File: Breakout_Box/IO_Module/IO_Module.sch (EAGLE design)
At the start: 5 parts, among them U1 AGND, U2 AGND, U3 AGND

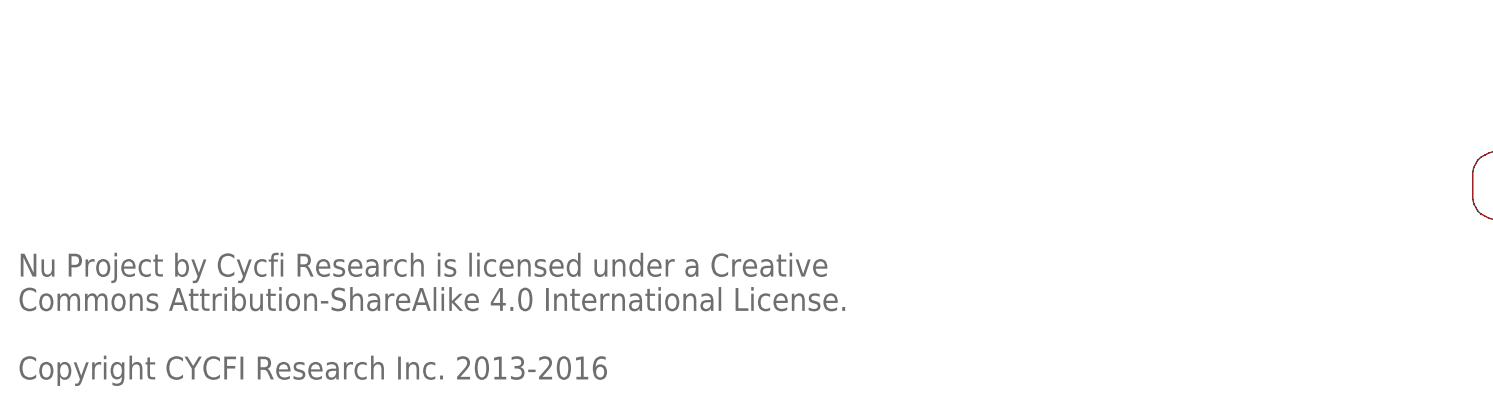
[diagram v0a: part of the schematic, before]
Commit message: Licenses
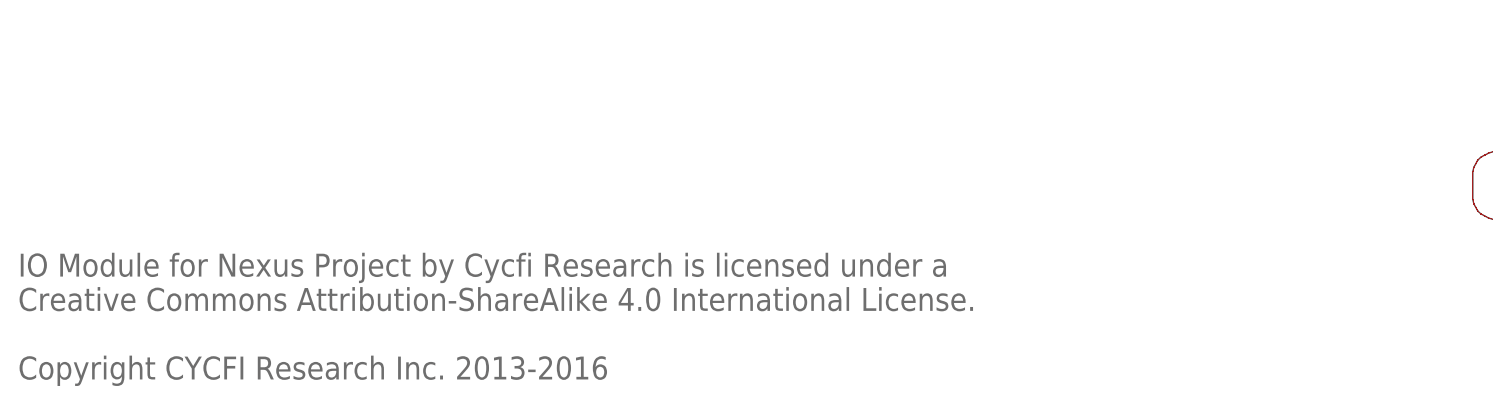
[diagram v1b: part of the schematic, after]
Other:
- note added: "IO Module for Nexus Project by Cycfi Research is licensed under a Creative Commons Attribution-ShareAlike 4.0 International License. Copyright CYCFI Research Inc. 2013-2016"
- note removed: "Nu Project by Cycfi Research is licensed under a Creative Commons Attribution-ShareAlike 4.0 International License. Copyright CYCFI Research Inc. 2013-2016"
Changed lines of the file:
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@@
 <wire x1="233.45903125" y1="25.186403125" x2="233.45903125" y2="33.142509375" width="0" layer="94"/>
 <text x="252.73" y="6.985" size="2.54" layer="95">v0.9</text>
-<text x="12.7" y="7.62" size="2.54" layer="95">Nu Project by Cycfi Research is licensed under a Creative
-Commons Attribution-ShareAlike 4.0 International License.
+<text x="12.7" y="7.62" size="2.54" layer="95">IO Module for Nexus Project by Cycfi Research is licensed under a
+Creative Commons Attribution-ShareAlike 4.0 International License.
 Copyright CYCFI Research Inc. 2013-2016</text>
 <text x="200.025" y="11.43" size="2.54" layer="95">2016050</text>

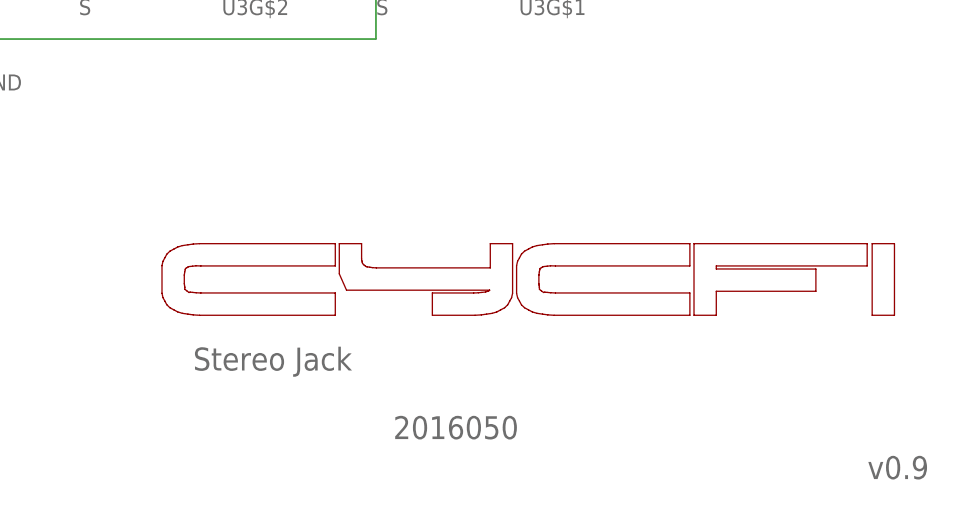
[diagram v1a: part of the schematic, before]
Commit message: *Edit Logo *Check BOM *Added 19P Connector Files
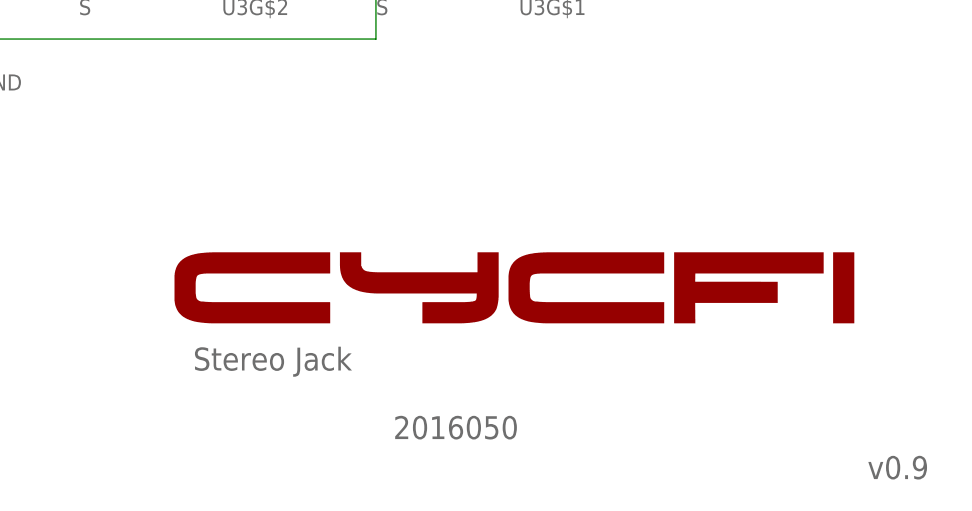
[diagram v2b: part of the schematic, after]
